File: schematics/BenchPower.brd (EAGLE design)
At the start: 79.7 x 67 mm, 28 parts, among them U1 V_REG_317SINK

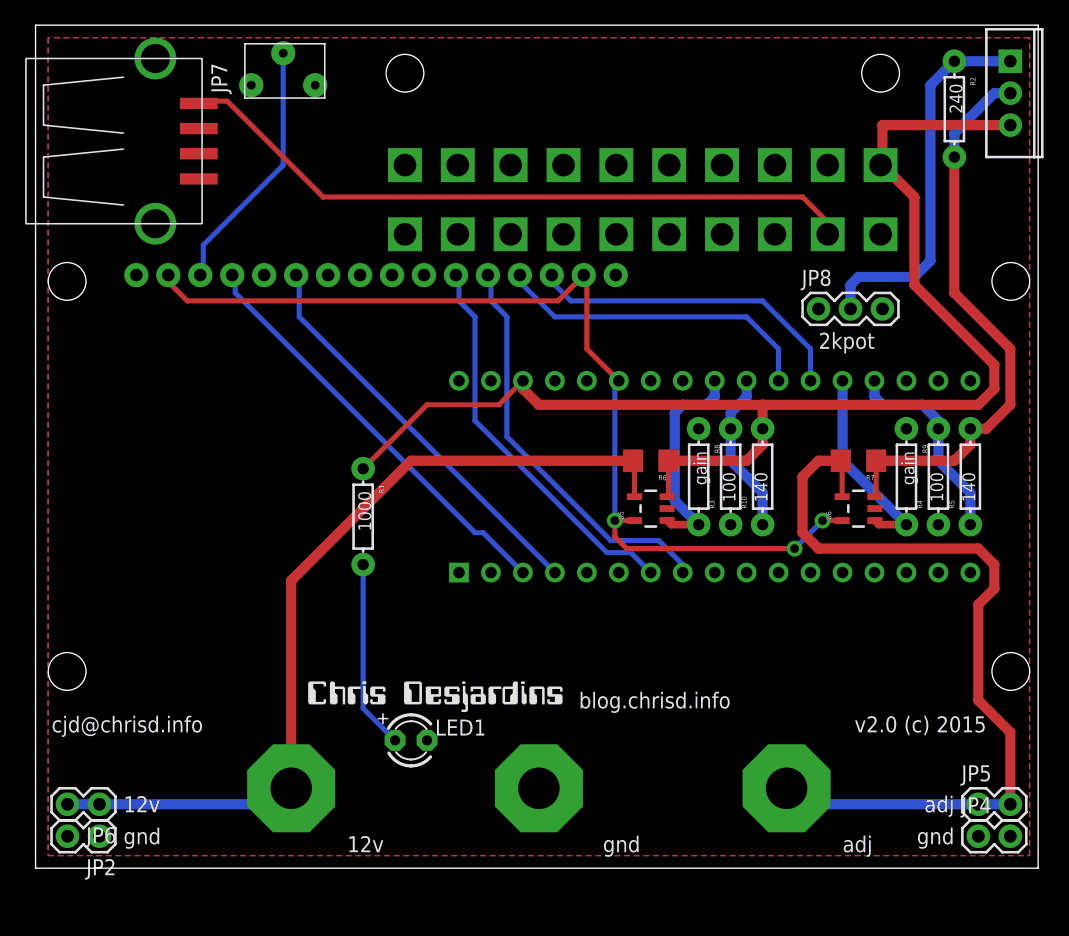
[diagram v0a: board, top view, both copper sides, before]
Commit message: New layout
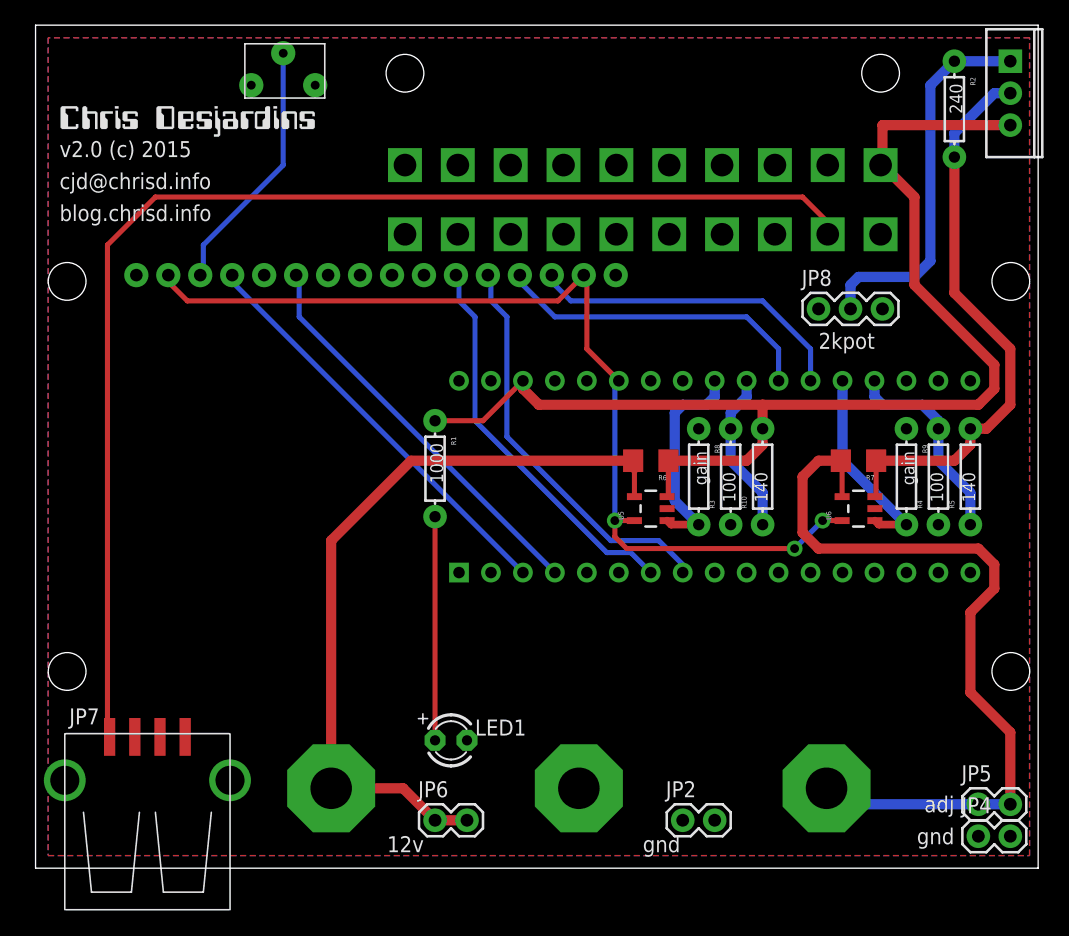
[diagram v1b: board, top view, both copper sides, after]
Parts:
- moved JP7 50.8 mm to (8.89, 6.99), turned to 90 degrees
- moved U$3 49.8 mm to (1.91, 58.7)
- moved JP2 46.4 mm to (51.4, 3.81), turned to 0 degrees
- moved JP6 26.7 mm to (31.8, 3.81), turned to 0 degrees
- moved R1 6.87 mm to (31.8, 31.8)
- moved LED1 3.18 mm to (33.0, 10.2)
- moved PWR1 3.18 mm to (62.9, 6.35)
- moved PWR2 3.18 mm to (23.5, 6.35)
- moved U$5 3.17 mm to (43.2, 6.35)
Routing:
- net 5VATX: track 55.1 -> 99.9 mm
- net AMPS12VHDR: track 68.8 -> 61.0 mm
- net 12VHDR: track 103.8 -> 96.6 mm
- net N$1: track 15.0 -> 17.8 mm
- net AMPS12VREG: track 66.1 -> 63.5 mm
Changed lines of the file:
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@@
 <wire x1="79.6825" y1="67" x2="0" y2="67" width="0" layer="20"/>
 <wire x1="0" y1="67" x2="0" y2="0" width="0" layer="20"/>
-<text x="1.27" y="10.795" size="1.27" layer="21" font="vector">cjd@chrisd.info</text>
-<text x="65.0875" y="10.795" size="1.27" layer="21" font="vector">v2.0 (c) 2015</text>
-<text x="64.135" y="1.27" size="1.27" layer="21" font="vector">adj</text>
-<text x="24.765" y="1.27" size="1.27" layer="21" font="vector">12v</text>
-<text x="43.18" y="12.7" size="1.27" layer="21" font="vector">blog.chrisd.info</text>
-<text x="45.085" y="1.27" size="1.27" layer="21" font="vector">gnd</text>
-<text x="6.985" y="4.445" size="1.27" layer="21" font="vector">12v</text>
-<text x="6.985" y="1.905" size="1.27" layer="21" font="vector">gnd</text>
+<text x="1.905" y="53.975" size="1.27" layer="21" font="vector">cjd@chrisd.info</text>
+<text x="1.905" y="56.515" size="1.27" layer="21" font="vector">v2.0 (c) 2015</text>
+<text x="27.94" y="1.27" size="1.27" layer="21" font="vector">12v</text>
+<text x="1.905" y="51.435" size="1.27" layer="21" font="vector">blog.chrisd.info</text>
+<text x="48.26" y="1.27" size="1.27" layer="21" font="vector">gnd</text>
 <text x="73.025" y="5.715" size="1.27" layer="21" font="vector" rot="R180">adj</text>
 <text x="73.025" y="3.175" size="1.27" layer="21" font="vector" rot="R180">gnd</text>
@@
 </autorouter>
 <elements>
-<element name="PWR1" library="desjardins" package="BINDINGPOST" value="BINDINGPOST" x="59.69" y="6.35"/>
-<element name="PWR2" library="desjardins" package="BINDINGPOST" value="BINDINGPOST" x="20.32" y="6.35"/>
-<element name="U$5" library="desjardins" package="BINDINGPOST" value="BINDINGPOST" x="40.005" y="6.35"/>
+<element name="PWR1" library="desjardins" package="BINDINGPOST" value="BINDINGPOST" x="62.865" y="6.35"/>
+<element name="PWR2" library="desjardins" package="BINDINGPOST" value="BINDINGPOST" x="23.495" y="6.35"/>
+<element name="U$5" library="desjardins" package="BINDINGPOST" value="BINDINGPOST" x="43.18" y="6.35"/>
 <element name="ATXCONN" library="desjardins" package="ATXPOWER" value="ATXPOWER" x="48.26" y="55.88" rot="R270"/>
 <element name="ARDUINOMICRO" library="ChrisD" package="ARDUINO_PRO_MICRO" value="ARDUINO_PRO_MICRO" x="78.105" y="22.225" rot="R90"/>
 <element name="U1" library="SparkFun-PowerIC" package="TO220-ADJ" value="V_REG_317SINK" x="77.47" y="61.595" rot="R270"/>
-<element name="R1" library="SparkFun-Passives" package="AXIAL-0.3" value="1000" x="26.035" y="27.94" rot="R270"/>
+<element name="R1" library="SparkFun-Passives" package="AXIAL-0.3" value="1000" x="31.75" y="31.75" rot="R270"/>
 <element name="R2" library="SparkFun-Passives" package="AXIAL-0.3" value="240" x="73.025" y="60.325" rot="R270"/>
-<element name="U$3" library="desjardins" package="LOGO" value="" x="21.59" y="13.0175"/>
+<element name="U$3" library="desjardins" package="LOGO" value="" x="1.905" y="58.7375"/>
 <element name="LCD" library="desjardins" package="DT162C" value="16X2LCDDT162C" x="40.01" y="31.135"/>
-<element name="LED1" library="adafruit" package="LED3MM" value="" x="29.845" y="10.16"/>
+<element name="LED1" library="adafruit" package="LED3MM" value="" x="33.02" y="10.16"/>
 <element name="R6" library="SparkFun-Resistors" package="1206" value="" x="48.895" y="32.385" rot="R180"/>
 <element name="R7" library="SparkFun-Resistors" package="1206" value="" x="65.405" y="32.385" rot="R180"/>
@@
 <element name="R8" library="SparkFun-Passives" package="AXIAL-0.3" value="gain" x="52.705" y="31.115" rot="R270"/>
 <element name="R9" library="SparkFun-Passives" package="AXIAL-0.3" value="gain" x="69.215" y="31.115" rot="R270"/>
-<element name="JP2" library="SparkFun-Connectors" package="1X02" value="M02PTH" x="5.08" y="2.54" rot="R180"/>
+<element name="JP2" library="SparkFun-Connectors" package="1X02" value="M02PTH" x="51.435" y="3.81"/>
 <element name="R3" library="SparkFun-Passives" package="AXIAL-0.3" value="100" x="55.245" y="31.115" rot="R90"/>
 <element name="R10" library="SparkFun-Passives" package="AXIAL-0.3" value="140" x="57.785" y="31.115" rot="R90"/>
 <element name="JP4" library="SparkFun-Connectors" package="1X02" value="M02PTH" x="74.93" y="2.54"/>
 <element name="JP5" library="SparkFun-Connectors" package="1X02" value="M02PTH" x="74.93" y="5.08"/>
-<element name="JP6" library="SparkFun-Connectors" package="1X02" value="M02PTH" x="5.08" y="5.08" rot="R180"/>
-<element name="JP7" library="SparkFun-Connectors" package="USB-A-S" value="USB-A-S" x="9.525" y="57.785"/>
+<element name="JP6" library="SparkFun-Connectors" package="1X02" value="M02PTH" x="31.75" y="3.81"/>
+<element name="JP7" library="SparkFun-Connectors" package="USB-A-S" value="USB-A-S" x="8.89" y="6.985" rot="R90"/>
 <element name="JP8" library="SparkFun-Connectors" package="1X03" value="" x="62.23" y="44.45"/>
 </elements>
@@
 <wire x1="40.005" y1="36.83" x2="57.785" y2="36.83" width="0.8128" layer="1"/>
 <wire x1="57.785" y1="36.83" x2="57.785" y2="34.925" width="0.8128" layer="1"/>
-<wire x1="31.115" y1="36.83" x2="36.83" y2="36.83" width="0.4064" layer="1"/>
-<wire x1="36.83" y1="36.83" x2="38.735" y2="38.735" width="0.4064" layer="1"/>
-<wire x1="31.115" y1="36.83" x2="26.035" y2="31.75" width="0.4064" layer="1"/>
+<wire x1="31.75" y1="35.56" x2="35.56" y2="35.56" width="0.4064" layer="1"/>
+<wire x1="35.56" y1="35.56" x2="38.735" y2="38.735" width="0.4064" layer="1"/>
 </signal>
 <signal name="N$1">
 <contactref element="R1" pad="P$2"/>
 <contactref element="LED1" pad="A"/>
-<wire x1="26.035" y1="24.13" x2="26.035" y2="12.7" width="0.4064" layer="16"/>
-<wire x1="26.035" y1="12.7" x2="28.575" y2="10.16" width="0.4064" layer="16"/>
+<wire x1="31.75" y1="27.94" x2="31.75" y2="10.16" width="0.4064" layer="1"/>
 </signal>
 <signal name="PWR_OK">
@@
 <wire x1="60.96" y1="26.67" x2="62.23" y2="25.4" width="0.8128" layer="1"/>
 <wire x1="62.23" y1="25.4" x2="74.93" y2="25.4" width="0.8128" layer="1"/>
-<wire x1="76.2" y1="22.225" x2="74.93" y2="20.955" width="0.8128" layer="1"/>
+<wire x1="76.2" y1="22.225" x2="74.295" y2="20.32" width="0.8128" layer="1"/>
 <wire x1="74.93" y1="5.08" x2="77.47" y2="5.08" width="0.8128" layer="16"/>
-<wire x1="74.93" y1="20.955" x2="74.93" y2="13.335" width="0.8128" layer="1"/>
-<wire x1="74.93" y1="13.335" x2="77.47" y2="10.795" width="0.8128" layer="1"/>
+<wire x1="74.295" y1="20.32" x2="74.295" y2="13.97" width="0.8128" layer="1"/>
+<wire x1="74.295" y1="13.97" x2="77.47" y2="10.795" width="0.8128" layer="1"/>
 <wire x1="77.47" y1="10.795" x2="77.47" y2="5.08" width="0.8128" layer="1"/>
-<wire x1="74.93" y1="5.08" x2="60.96" y2="5.08" width="0.8128" layer="16"/>
-<wire x1="60.96" y1="5.08" x2="59.69" y2="6.35" width="0.8128" layer="16"/>
+<wire x1="74.93" y1="5.08" x2="64.135" y2="5.08" width="0.8128" layer="16"/>
+<wire x1="64.135" y1="5.08" x2="62.865" y2="6.35" width="0.8128" layer="16"/>
 </signal>
 <signal name="AMPS12VHDR">
@@
 <wire x1="47.5949" y1="29.525" x2="47.5949" y2="31.6501" width="0.4064" layer="1"/>
 <wire x1="47.5949" y1="31.6501" x2="47.495" y2="32.385" width="0.6096" layer="1"/>
-<wire x1="20.32" y1="22.86" x2="20.32" y2="6.35" width="0.8128" layer="1"/>
-<wire x1="20.32" y1="22.86" x2="29.845" y2="32.385" width="0.8128" layer="1"/>
 <wire x1="29.845" y1="32.385" x2="47.495" y2="32.385" width="0.8128" layer="1"/>
 <contactref element="JP6" pad="2"/>
 <contactref element="JP6" pad="1"/>
-<wire x1="2.54" y1="5.08" x2="5.08" y2="5.08" width="0.8128" layer="16"/>
-<wire x1="5.08" y1="5.08" x2="19.05" y2="5.08" width="0.8128" layer="16"/>
-<wire x1="19.05" y1="5.08" x2="20.32" y2="6.35" width="0.8128" layer="16"/>
+<wire x1="29.845" y1="32.385" x2="23.495" y2="26.035" width="0.8128" layer="1"/>
+<wire x1="23.495" y1="26.035" x2="23.495" y2="6.35" width="0.8128" layer="1"/>
+<wire x1="23.495" y1="6.35" x2="29.21" y2="6.35" width="0.8128" layer="1"/>
+<wire x1="29.21" y1="6.35" x2="31.75" y2="3.81" width="0.8128" layer="1"/>
+<wire x1="31.75" y1="3.81" x2="34.29" y2="3.81" width="0.8128" layer="1"/>
 </signal>
 <signal name="3.3V$2">
@@
 <contactref element="LCD" pad="P$4"/>
 <contactref element="ARDUINOMICRO" pad="P3"/>
-<wire x1="35.56" y1="26.67" x2="38.735" y2="23.495" width="0.4064" layer="16"/>
-<wire x1="35.56" y1="26.67" x2="34.925" y2="26.67" width="0.4064" layer="16"/>
-<wire x1="34.925" y1="26.67" x2="15.875" y2="45.72" width="0.4064" layer="16"/>
-<wire x1="15.875" y1="45.72" x2="15.875" y2="46.89" width="0.4064" layer="16"/>
-<wire x1="15.875" y1="46.89" x2="15.63" y2="47.135" width="0.4064" layer="16"/>
+<wire x1="38.735" y1="23.495" x2="15.63" y2="46.6" width="0.4064" layer="16"/>
+<wire x1="15.63" y1="46.6" x2="15.63" y2="47.135" width="0.4064" layer="16"/>
 </signal>
 <signal name="LCD_EN">
@@
 <wire x1="62.865" y1="51.435" x2="62.865" y2="50.475" width="0.4064" layer="1"/>
 <wire x1="62.865" y1="50.475" x2="62.96" y2="50.38" width="0.4064" layer="1"/>
-<wire x1="60.96" y1="53.34" x2="22.86" y2="53.34" width="0.4064" layer="1"/>
-<wire x1="22.86" y1="53.34" x2="15.24" y2="60.96" width="0.4064" layer="1"/>
-<wire x1="15.24" y1="60.96" x2="13.15" y2="60.96" width="0.4064" layer="1"/>
-<wire x1="13.15" y1="60.96" x2="12.975" y2="60.785" width="0.4064" layer="1"/>
+<wire x1="60.96" y1="53.34" x2="9.525" y2="53.34" width="0.4064" layer="1"/>
+<wire x1="9.525" y1="53.34" x2="5.715" y2="49.53" width="0.4064" layer="1"/>
+<wire x1="5.715" y1="49.53" x2="5.715" y2="10.61" width="0.4064" layer="1"/>
+<wire x1="5.715" y1="10.61" x2="5.89" y2="10.435" width="0.4064" layer="1"/>
 </signal>
 <signal name="5V$4">
